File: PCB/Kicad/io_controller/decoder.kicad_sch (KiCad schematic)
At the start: 26 parts

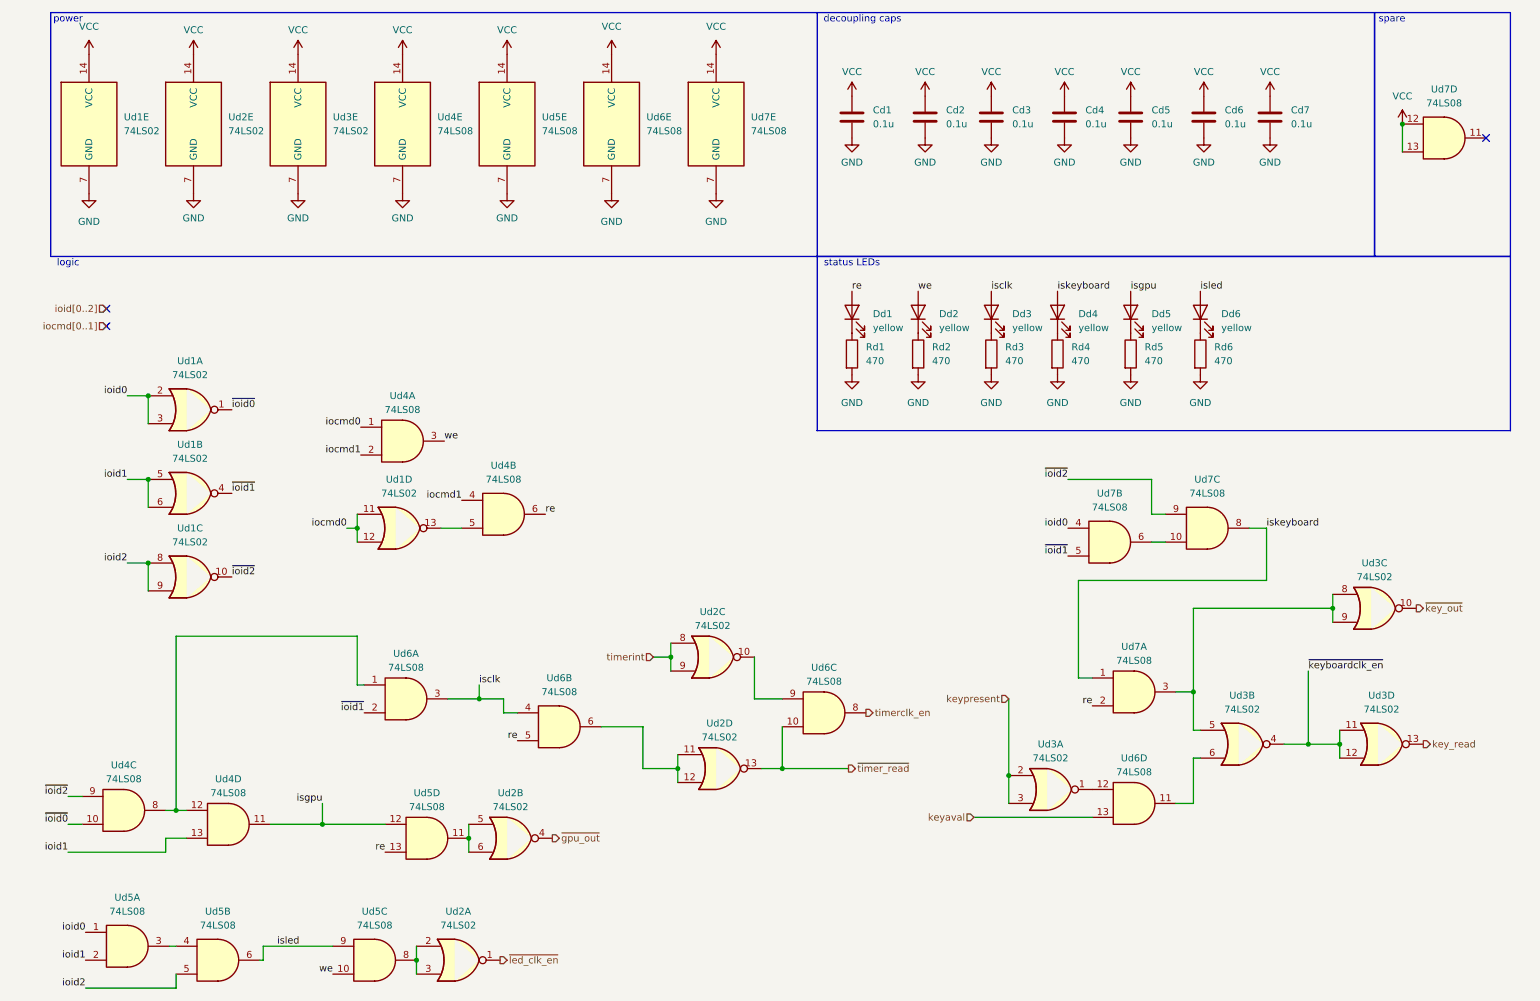
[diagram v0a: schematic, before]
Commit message: primarily keyboard decoder finish ; preliminary layout
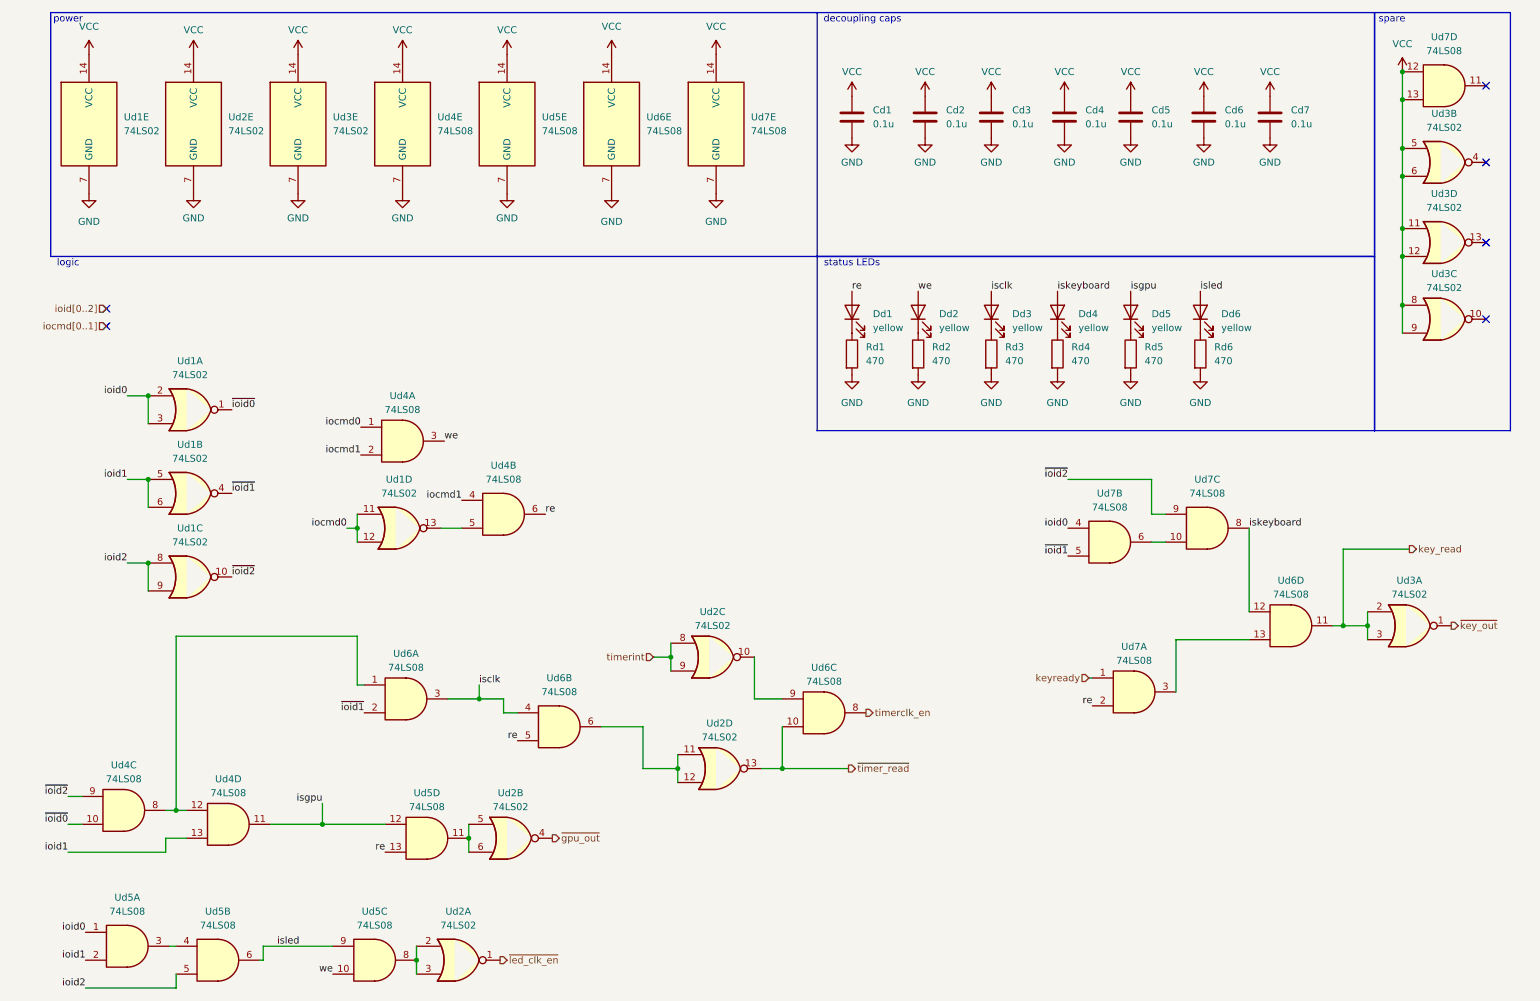
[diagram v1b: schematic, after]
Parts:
- Ud3: footprint (none) -> Package_SO:SO-14_3.9x8.65mm_P1.27mm
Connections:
- net keypresent is gone; now on net key_read: Ud3.2, Ud3.3
- net VCC: now also Ud3.11, Ud3.12, Ud3.5, Ud3.6, Ud3.8, Ud3.9
- net iskeyboard: now also Ud6.12; no longer Ud7.1
- net key_read: now also Ud6.11; no longer Ud3.13
- net ~{key_out}: now also Ud3.1; no longer Ud3.10
- net keyaval: no longer names the net of Ud6.13
- net keyaval: now also Ud7.3
- removed net ~{keyboardclk_en}: Ud3.11, Ud3.12, Ud3.4
- new net keyready: Ud7.1
- no-connect marks 3 -> 6
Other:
- moved on the sheet: Ud3A, Ud3B, Ud3C, Ud3D, Ud6D, Ud7D
